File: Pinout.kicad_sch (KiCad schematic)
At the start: 4 parts, among them J7 Conn_01x02_Pin, J8 Conn_01x02_Pin

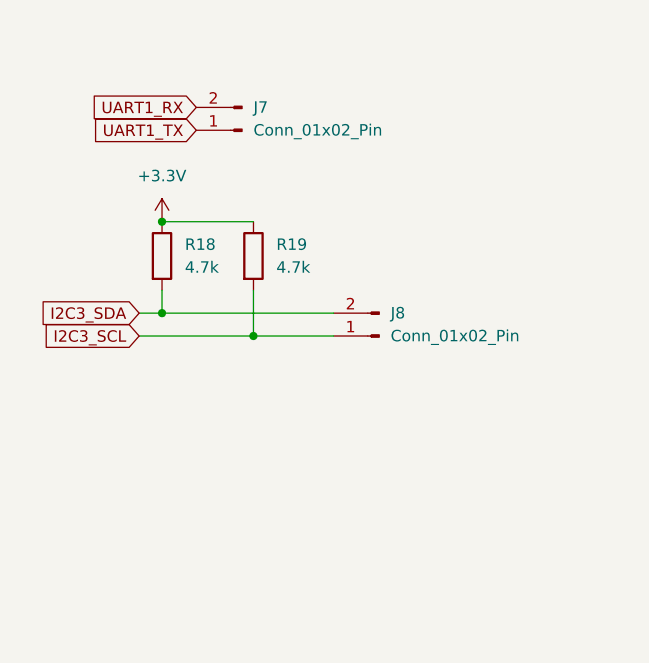
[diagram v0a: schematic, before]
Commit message: "Update KiRA Flight Computer schematic and PCB files"
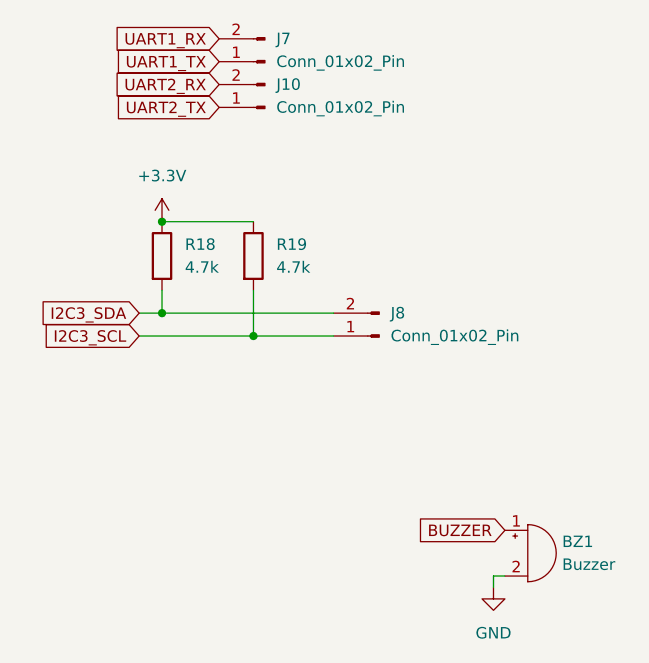
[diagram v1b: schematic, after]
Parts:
- added BZ1: Buzzer, symbol Device:Buzzer
- added J10: Conn_01x02_Pin, Connector_PinHeader_2.54mm:PinHeader_1x02_P2.54mm_Vertical, symbol Connector:Conn_01x02_Pin
- J7, J8: footprint (none) -> Connector_PinHeader_2.54mm:PinHeader_1x02_P2.54mm_Vertical
- R18, R19: footprint (none) -> Resistor_SMD:R_0603_1608Metric
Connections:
- new net BUZZER: BZ1.1 (+)
- new net GND: BZ1.2 (-)
- new net UART2_RX: J10.2 (Pin_2)
- new net UART2_TX: J10.1 (Pin_1)
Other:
- moved on the sheet: J7

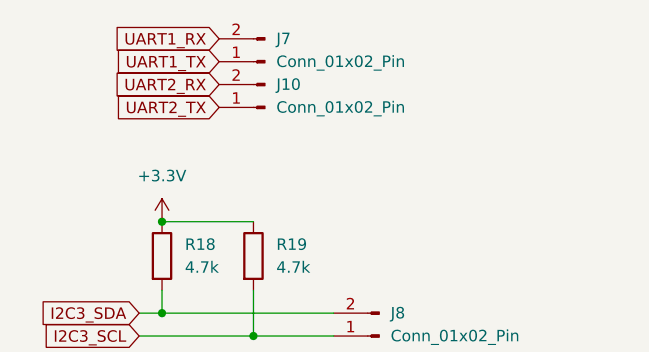
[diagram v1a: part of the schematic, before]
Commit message: Update PCB
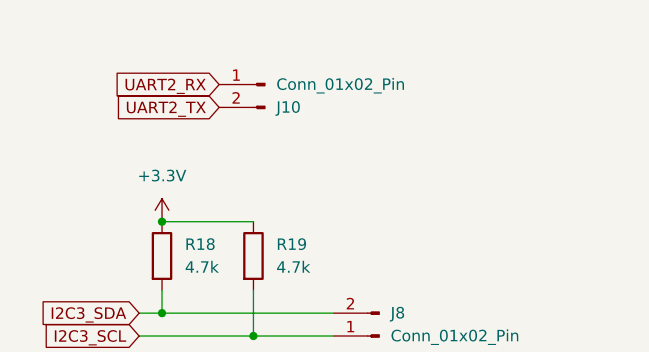
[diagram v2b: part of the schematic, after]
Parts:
- removed J7: Conn_01x02_Pin, Connector_PinHeader_2.54mm:PinHeader_1x02_P2.54mm_Vertical, symbol Connector:Conn_01x02_Pin
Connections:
- net UART2_RX: now also J10.1 (Pin_1); no longer J10.2 (Pin_2)
- net UART2_TX: now also J10.2 (Pin_2); no longer J10.1 (Pin_1)
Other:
- moved on the sheet: J10
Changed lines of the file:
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@@
 		)
 	)
-	(global_label "UART1_RX"
+	(global_label "I2C3_SCL"
 		(shape input)
-		(at 48.26 36.83 180)
+		(at 39.37 69.85 180)
 		(fields_autoplaced yes)
 		(effects
@@
 		)
 		(property "Intersheetrefs" "${INTERSHEET_REFS}"
-			(at 35.9615 36.83 0)
-			(effects
-				(font
-					(size 1.27 1.27)
-				)
-				(justify right)
-				(hide yes)
-			)
-		)
-	)
-	(global_label "UART1_TX"
+			(at 27.6158 69.85 0)
+			(effects
+				(font
+					(size 1.27 1.27)
+				)
+				(justify right)
+				(hide yes)
+			)
+		)
+	)
+	(global_label "I2C3_SDA"
 		(shape input)
-		(at 48.26 39.37 180)
+		(at 39.37 67.31 180)
 		(fields_autoplaced yes)
 		(effects
@@
 		)
 		(property "Intersheetrefs" "${INTERSHEET_REFS}"
-			(at 36.2639 39.37 0)
-			(effects
-				(font
-					(size 1.27 1.27)
-				)
-				(justify right)
-				(hide yes)
-			)
-		)
-	)
-	(global_label "I2C3_SCL"
+			(at 27.5553 67.31 0)
+			(effects
+				(font
+					(size 1.27 1.27)
+				)
+				(justify right)
+				(hide yes)
+			)
+		)
+	)
+	(global_label "UART2_RX"
 		(shape input)
-		(at 39.37 69.85 180)
+		(at 48.26 41.91 180)
 		(fields_autoplaced yes)
 		(effects
@@
 		)
 		(property "Intersheetrefs" "${INTERSHEET_REFS}"
-			(at 27.6158 69.85 0)
-			(effects
-				(font
-					(size 1.27 1.27)
-				)
-				(justify right)
-				(hide yes)
-			)
-		)
-	)
-	(global_label "I2C3_SDA"
+			(at 35.9615 41.91 0)
+			(effects
+				(font
+					(size 1.27 1.27)
+				)
+				(justify right)
+				(hide yes)
+			)
+		)
+	)
+	(global_label "UART2_TX"
 		(shape input)
-		(at 39.37 67.31 180)
+		(at 48.26 44.45 180)
 		(fields_autoplaced yes)
 		(effects
@@
 		)
 		(property "Intersheetrefs" "${INTERSHEET_REFS}"
-			(at 27.5553 67.31 0)
-			(effects
-				(font
-					(size 1.27 1.27)
-				)
-				(justify right)
-				(hide yes)
-			)
-		)
-	)
-	(global_label "UART2_RX"
-		(shape input)
-		(at 48.26 41.91 180)
-		(fields_autoplaced yes)
-		(effects
-			(font
-				(size 1.27 1.27)
-			)
-			(justify right)
-		)
-		(property "Intersheetrefs" "${INTERSHEET_REFS}"
-			(at 35.9615 41.91 0)
-			(effects
-				(font
-					(size 1.27 1.27)
-				)
-				(justify right)
-				(hide yes)
-			)
-		)
-	)
-	(global_label "UART2_TX"
-		(shape input)
-		(at 48.26 44.45 180)
-		(fields_autoplaced yes)
-		(effects
-			(font
-				(size 1.27 1.27)
-			)
-			(justify right)
-		)
-		(property "Intersheetrefs" "${INTERSHEET_REFS}"
 			(at 36.2639 44.45 0)
 			(effects
@@
 	(symbol
 		(lib_id "Connector:Conn_01x02_Pin")
-		(at 53.34 39.37 180)
-		(unit 1)
-		(exclude_from_sim no)
-		(in_bom yes)
-		(on_board yes)
-		(dnp no)
-		(fields_autoplaced yes)
-		(property "Reference" "J7"
-			(at 54.61 36.8299 0)
+		(at 53.34 41.91 0)
+		(mirror y)
+		(unit 1)
+		(exclude_from_sim no)
+		(in_bom yes)
+		(on_board yes)
+		(dnp no)
+		(property "Reference" "J10"
+			(at 54.61 44.4501 0)
 			(effects
 				(font
@@
 		)
 		(property "Value" "Conn_01x02_Pin"
-			(at 54.61 39.3699 0)
+			(at 54.61 41.9101 0)
 			(effects
 				(font
@@
 		)
 		(property "Footprint" "Connector_PinHeader_2.54mm:PinHeader_1x02_P2.54mm_Vertical"
-			(at 53.34 39.37 0)
+			(at 53.34 41.91 0)
 			(effects
 				(font
@@
 		)
 		(property "Datasheet" "~"
-			(at 53.34 39.37 0)
+			(at 53.34 41.91 0)
 			(effects
 				(font
@@
 		)
 		(property "Description" "Generic connector, single row, 01x02, script generated"
-			(at 53.34 39.37 0)
-			(effects
-				(font
-					(size 1.27 1.27)
-				)
-				(hide yes)
-			)
-		)
-		(pin "1"
-		)
-		(pin "2"
-		)
-		(instances
-			(project ""
-				(path "/aff8106b-a9b7-4e48-85ad-25b2eb3ce379/b67f38d8-38f4-48c0-8f3f-0b1ef1ce702f"
-					(reference "J7")
-					(unit 1)
-				)
-			)
-		)
-	)
-	(symbol
-		(lib_id "Connector:Conn_01x02_Pin")
-		(at 53.34 44.45 180)
-		(unit 1)
-		(exclude_from_sim no)
-		(in_bom yes)
-		(on_board yes)
-		(dnp no)
-		(fields_autoplaced yes)
-		(property "Reference" "J10"
-			(at 54.61 41.9099 0)
-			(effects
-				(font
-					(size 1.27 1.27)
-				)
-				(justify right)
-			)
-		)
-		(property "Value" "Conn_01x02_Pin"
-			(at 54.61 44.4499 0)
-			(effects
-				(font
-					(size 1.27 1.27)
-				)
-				(justify right)
-			)
-		)
-		(property "Footprint" "Connector_PinHeader_2.54mm:PinHeader_1x02_P2.54mm_Vertical"
-			(at 53.34 44.45 0)
-			(effects
-				(font
-					(size 1.27 1.27)
-				)
-				(hide yes)
-			)
-		)
-		(property "Datasheet" "~"
-			(at 53.34 44.45 0)
-			(effects
-				(font
-					(size 1.27 1.27)
-				)
-				(hide yes)
-			)
-		)
-		(property "Description" "Generic connector, single row, 01x02, script generated"
-			(at 53.34 44.45 0)
+			(at 53.34 41.91 0)
 			(effects
 				(font
@@
 		(on_board yes)
 		(dnp no)
-		(fields_autoplaced yes)
 		(property "Reference" "J8"
 			(at 67.31 67.3099 0)

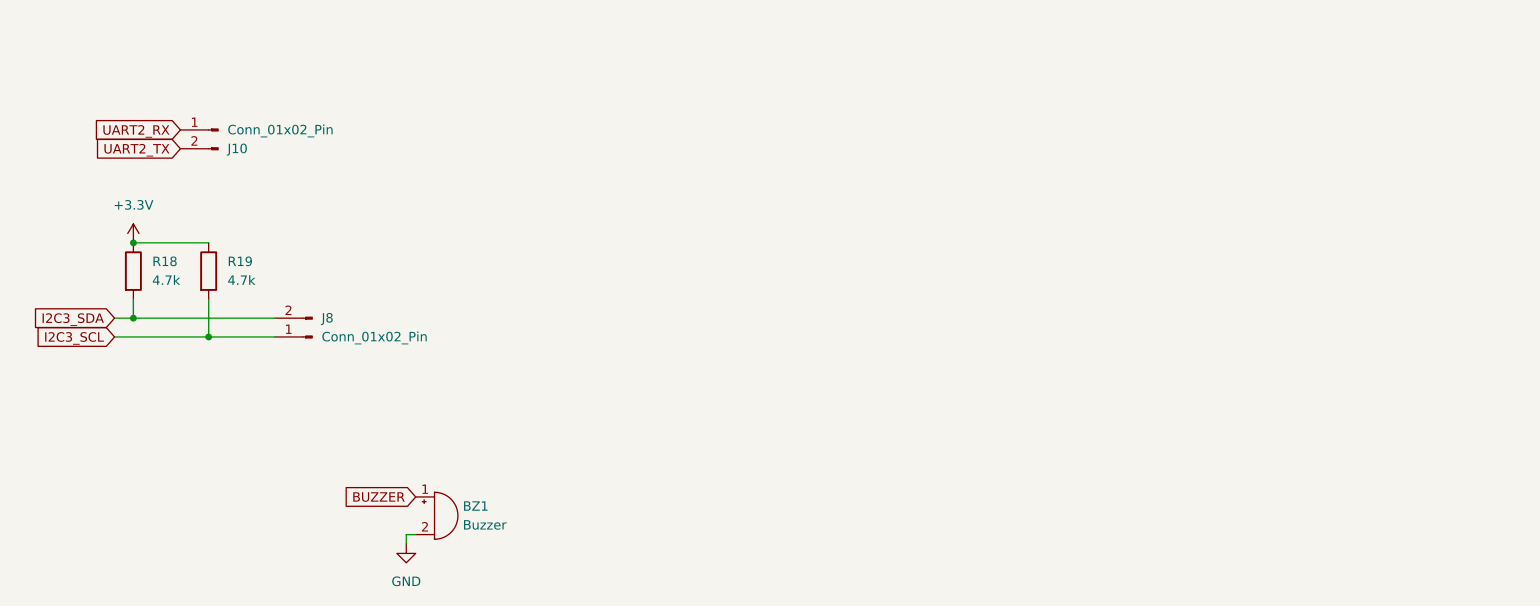
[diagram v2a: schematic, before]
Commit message: Update PCB
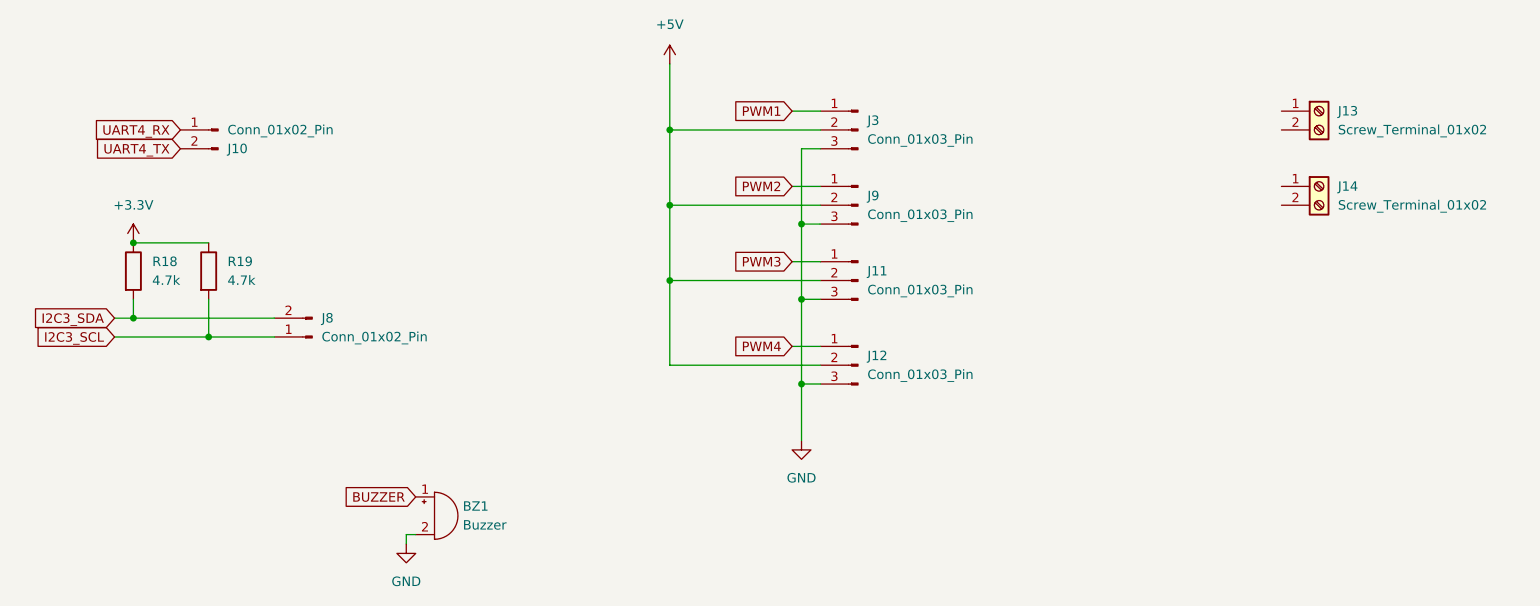
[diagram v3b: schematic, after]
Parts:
- added J11, J12, J3, J9: Conn_01x03_Pin, Connector_PinHeader_2.54mm:PinHeader_1x03_P2.54mm_Vertical, symbol Connector:Conn_01x03_Pin
- added J13, J14: Screw_Terminal_01x02, TerminalBlock_Phoenix:TerminalBlock_Phoenix_MPT-0,5-2-2.54_1x02_P2.54mm_Horizontal, symbol Connector:Screw_Terminal_01x02
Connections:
- net GND: now also J11.3 (Pin_3), J12.3 (Pin_3), J3.3 (Pin_3), J9.3 (Pin_3)
- net UART2_RX renamed UART4_RX
- net UART2_TX renamed UART4_TX
- new net +5V: J11.2 (Pin_2), J12.2 (Pin_2), J3.2 (Pin_2), J9.2 (Pin_2)
- new net PWM1: J3.1 (Pin_1)
- new net PWM2: J9.1 (Pin_1)
- new net PWM3: J11.1 (Pin_1)
- new net PWM4: J12.1 (Pin_1)
